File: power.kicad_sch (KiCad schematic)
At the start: 12 parts, among them J1 USB4215-03-A, U3 NCP1117 3.3, U4 USBLC6-2SC6

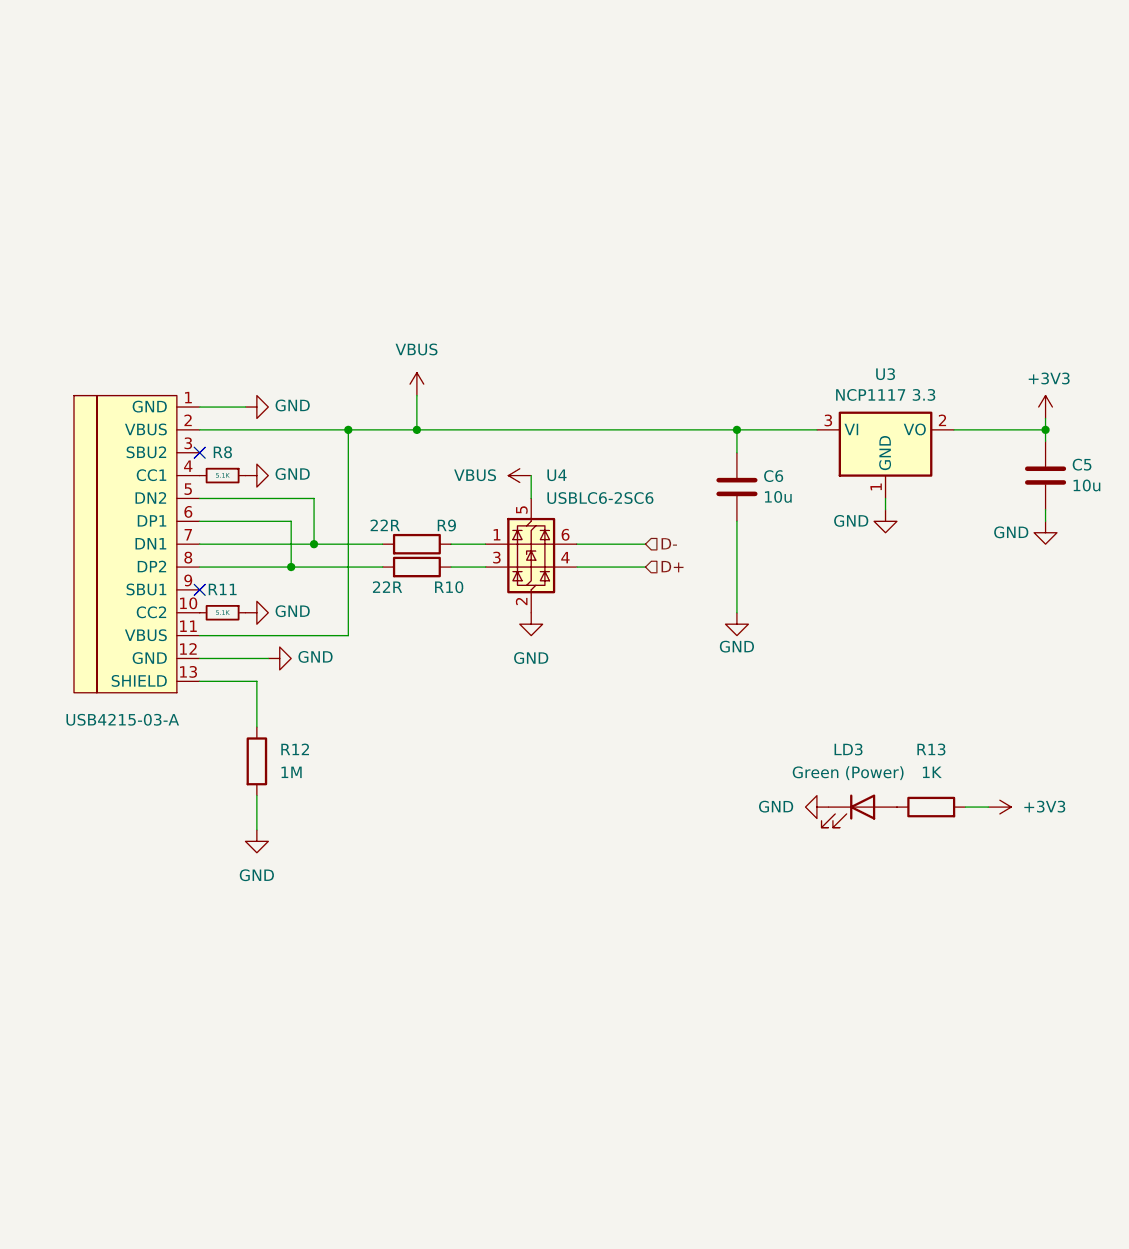
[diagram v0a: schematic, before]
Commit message: WIP
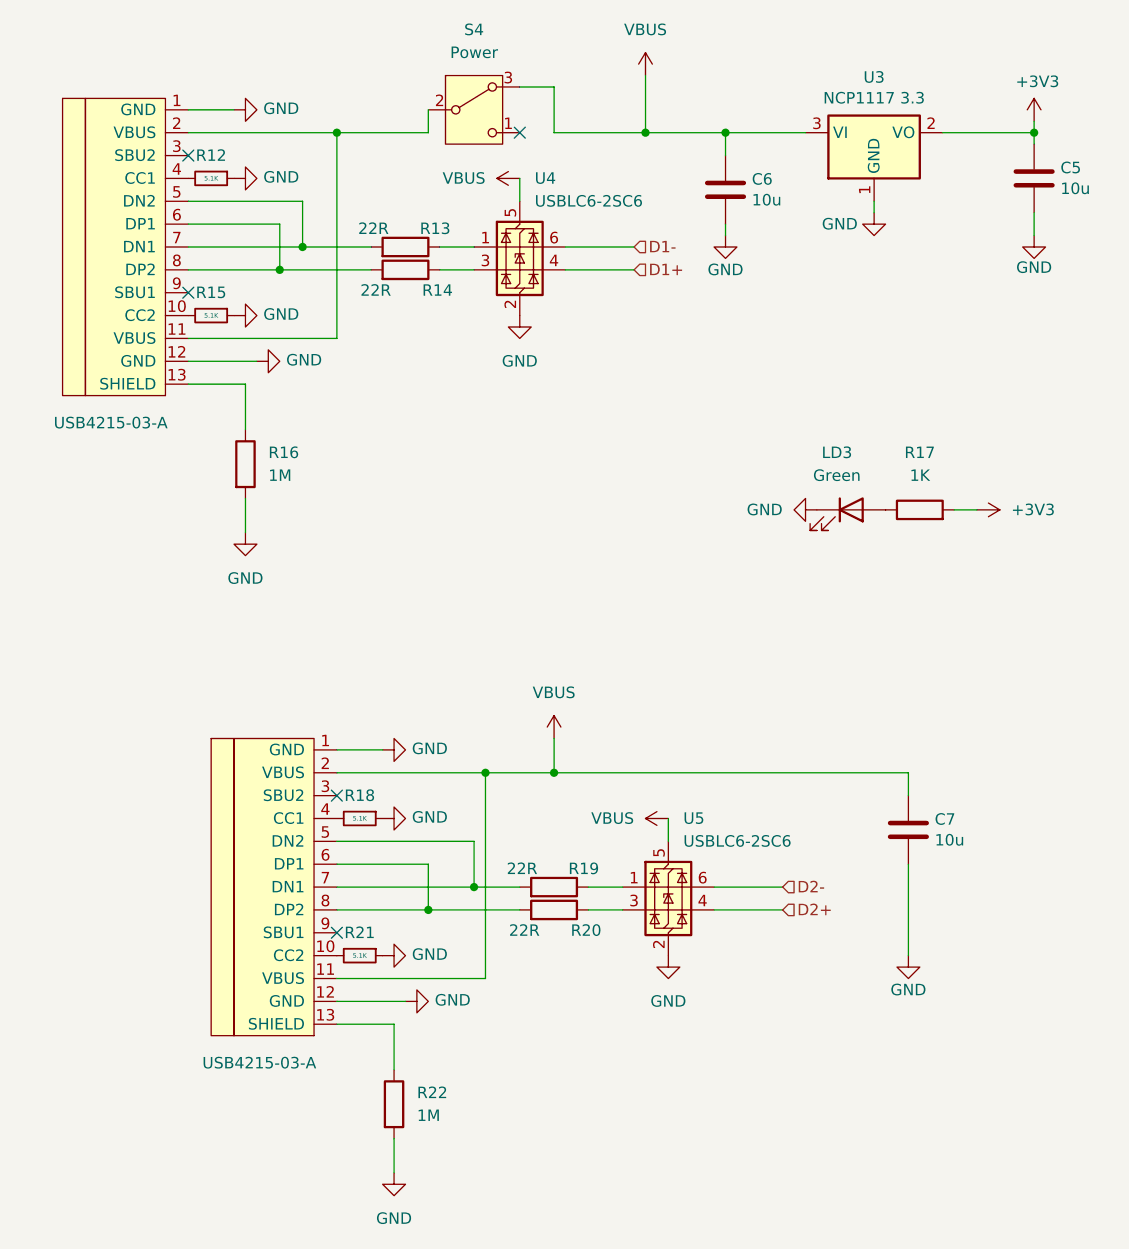
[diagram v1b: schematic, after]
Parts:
- added C7: 10u, FRANK:Capacitor (0805), symbol Device:C
- added J2: USB4215-03-A, FRANK:USB Type C, symbol FRANK:USB-C
- added R18, R21: 5.1K, FRANK:Resistor (0805), symbol Device:R_Small
- added R19, R20: 22R, FRANK:Resistor (0805), symbol Device:R
- added R22: 1M, FRANK:Resistor (0805), symbol Device:R
- added S4: Power, FRANK:Switch (MSK12C02), symbol Switch:SW_SPDT_321
- added U5: USBLC6-2SC6, FRANK:SOT-23-6, symbol Power_Protection:USBLC6-2SC6
- LD3: value Green (Power) -> Green
- U4: symbol Power_Protection:USBLC6-2SC6 -> FRANK:USBLC6-2SC6; AliExpress (none) -> https://vi.aliexpress.com/item/1005006883533480.html
- renumbered R8 to R12, R9 to R13, R10 to R14, R11 to R15, R12 to R16, R13 to R17
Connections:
- net GND: now also C7.2, J2.1 (GND), J2.12 (GND), R18.1, R21.1, R22.2, U5.2 (GND)
- net VBUS: now also C7.1, J2.11 (VBUS), J2.2 (VBUS), S4.3 (A), U5.5 (VBUS); no longer J1.11 (VBUS), J1.2 (VBUS)
- net D+ renamed D1+
- net D- renamed D1-
- new net: J1.11 (VBUS), J1.2 (VBUS), S4.2 (B)
- new net: J2.13 (SHIELD), R22.1
- new net: J2.4 (CC1), R18.2
- new net: R19.1, U5.1 (I/O1)
- new net: R20.1, U5.3 (I/O2)
- new net: J2.5 (DN2), J2.7 (DN1), R19.2
- new net: J2.6 (DP1), J2.8 (DP2), R20.2
- new net: J2.10 (CC2), R21.2
- new net D2+: U5.4 (I/O2)
- new net D2-: U5.6 (I/O1)
- no-connect marks 2 -> 5
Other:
- moved on the sheet: C5, C6, LD3, R12, R13, R14, R15, R16, R17, U3, U4

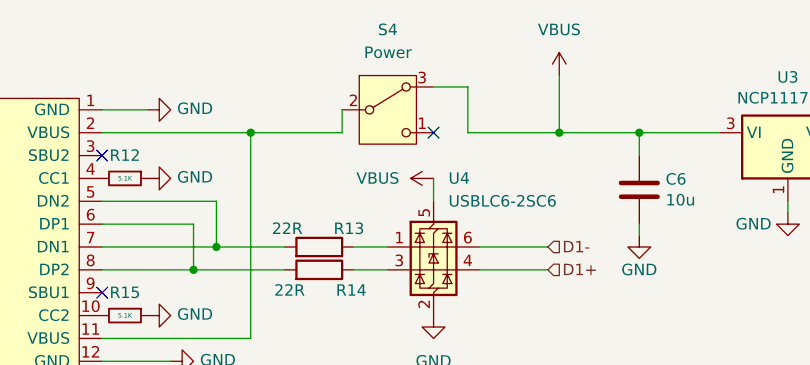
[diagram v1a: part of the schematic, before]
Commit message: Rev 1.05 WIP
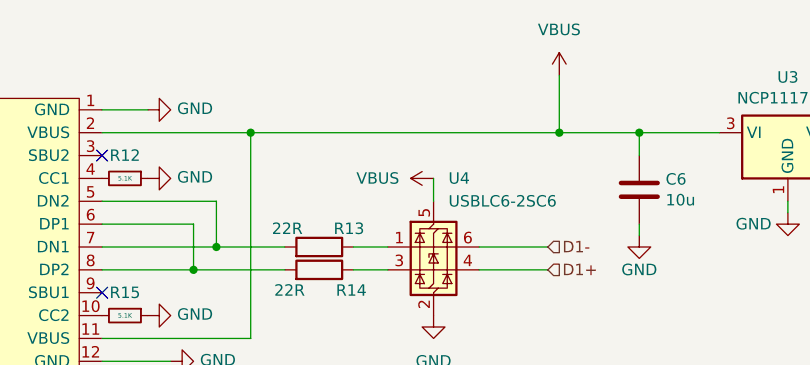
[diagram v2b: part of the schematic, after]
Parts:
- removed S4: Power, FRANK:Switch (MSK12C02), symbol Switch:SW_SPDT_321
- C5, C6, C7: footprint FRANK:Capacitor (0805) -> FRANK:Capacitor (0603)
- R12, R13, R14, R15, R16, R17, R18, R19, R20, R21, R22: footprint FRANK:Resistor (0805) -> FRANK:Resistor (0603)
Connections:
- net VBUS: now also J1.11 (VBUS), J1.2 (VBUS)
- no-connect marks 5 -> 4
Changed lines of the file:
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@@
 	)
 	(no_connect
-		(at 147.32 44.45)
-	)
-	(no_connect
 		(at 110.49 62.23)
 	)
@@
 	(wire
 		(pts
-			(xy 151.13 39.37) (xy 151.13 44.45)
-		)
-		(stroke
-			(width 0)
-			(type default)
-		)
-	)
-	(wire
-		(pts
 			(xy 163.83 120.65) (xy 163.83 123.19)
 		)
@@
 	(wire
 		(pts
-			(xy 127 44.45) (xy 137.16 44.45)
+			(xy 127 44.45) (xy 161.29 44.45)
 		)
 		(stroke
@@
 	(wire
 		(pts
-			(xy 151.13 44.45) (xy 161.29 44.45)
-		)
-		(stroke
-			(width 0)
-			(type default)
-		)
-	)
-	(wire
-		(pts
 			(xy 127 128.27) (xy 142.24 128.27)
 		)
@@
 	(wire
 		(pts
-			(xy 137.16 41.91) (xy 137.16 44.45)
-		)
-		(stroke
-			(width 0)
-			(type default)
-		)
-	)
-	(wire
-		(pts
 			(xy 168.91 128.27) (xy 176.53 128.27)
 		)
@@
 	(wire
 		(pts
-			(xy 147.32 39.37) (xy 151.13 39.37)
-		)
-		(stroke
-			(width 0)
-			(type default)
-		)
-	)
-	(wire
-		(pts
 			(xy 186.69 52.07) (xy 186.69 53.34)
 		)
@@
 	)
 	(symbol
-		(lib_id "Switch:SW_SPDT_321")
-		(at 142.24 41.91 0)
-		(unit 1)
-		(exclude_from_sim no)
-		(in_bom yes)
-		(on_board yes)
-		(dnp no)
-		(fields_autoplaced yes)
-		(property "Reference" "S4"
-			(at 142.24 33.02 0)
-			(effects
-				(font
-					(size 1.27 1.27)
-				)
-			)
-		)
-		(property "Value" "Power"
-			(at 142.24 35.56 0)
-			(effects
-				(font
-					(size 1.27 1.27)
-				)
-			)
-		)
-		(property "Footprint" "FRANK:Switch (MSK12C02)"
-			(at 142.24 52.07 0)
-			(effects
-				(font
-					(size 1.27 1.27)
-				)
-				(hide yes)
-			)
-		)
-		(property "Datasheet" "https://parts4laptops.eu/en/microbuttons/3300-microbutton-tact-switch-ts-1233-33x33x15mm-smt-mounting.html"
-			(at 142.24 49.53 0)
-			(effects
-				(font
-					(size 1.27 1.27)
-				)
-				(hide yes)
-			)
-		)
-		(property "Description" "Switch, single pole double throw"
-			(at 142.24 41.91 0)
-			(effects
-				(font
-					(size 1.27 1.27)
-				)
-				(hide yes)
-			)
-		)
-		(pin "2"
-		)
-		(pin "1"
-		)
-		(pin "3"
-		)
-		(instances
-			(project "echo"
-				(path "/8c0b3d8b-46d3-4173-ab1e-a61765f77d61/4ea27ee4-1edc-4e10-ab5a-91b9933087c0"
-					(reference "S4")
-					(unit 1)
-				)
-			)
-		)
-	)
-	(symbol
 		(lib_name "GND_5")
 		(lib_id "power:GND")
@@
 			)
 		)
-		(property "Footprint" "FRANK:Resistor (0805)"
+		(property "Footprint" "FRANK:Resistor (0603)"
 			(at 131.572 152.4 90)
 			(effects
@@
 			)
 		)
-		(property "Footprint" "FRANK:Capacitor (0805)"
+		(property "Footprint" "FRANK:Capacitor (0603)"
 			(at 191.4652 125.73 0)
 			(effects
@@
 			)
 		)
-		(property "Footprint" "FRANK:Resistor (0805)"
+		(property "Footprint" "FRANK:Resistor (0603)"
 			(at 134.62 58.928 90)
 			(effects
@@
 			)
 		)
-		(property "Footprint" "FRANK:Resistor (0805)"
+		(property "Footprint" "FRANK:Resistor (0603)"
 			(at 129.54 120.65 0)
 			(effects
@@
 			)
 		)
-		(property "Footprint" "FRANK:Capacitor (0805)"
+		(property "Footprint" "FRANK:Capacitor (0603)"
 			(at 205.4352 53.34 0)
 			(effects
@@
 			)
 		)
-		(property "Footprint" "FRANK:Capacitor (0805)"
+		(property "Footprint" "FRANK:Capacitor (0603)"
 			(at 171.1452 54.61 0)
 			(effects
@@
 			)
 		)
-		(property "Footprint" "FRANK:Resistor (0805)"
+		(property "Footprint" "FRANK:Resistor (0603)"
 			(at 191.77 88.138 90)
 			(effects
@@
 			)
 		)
-		(property "Footprint" "FRANK:Resistor (0805)"
+		(property "Footprint" "FRANK:Resistor (0603)"
 			(at 113.03 64.77 0)
 			(effects
@@
 			)
 		)
-		(property "Footprint" "FRANK:Resistor (0805)"
+		(property "Footprint" "FRANK:Resistor (0603)"
 			(at 113.03 49.53 0)
 			(effects
@@
 			)
 		)
-		(property "Footprint" "FRANK:Resistor (0805)"
+		(property "Footprint" "FRANK:Resistor (0603)"
 			(at 134.62 61.468 90)
 			(effects
@@
 			)
 		)
-		(property "Footprint" "FRANK:Resistor (0805)"
+		(property "Footprint" "FRANK:Resistor (0603)"
 			(at 151.13 130.048 90)
 			(effects
@@
 			)
 		)
-		(property "Footprint" "FRANK:Resistor (0805)"
+		(property "Footprint" "FRANK:Resistor (0603)"
 			(at 151.13 132.588 90)
 			(effects
@@
 			)
 		)
-		(property "Footprint" "FRANK:Resistor (0805)"
+		(property "Footprint" "FRANK:Resistor (0603)"
 			(at 115.062 81.28 90)
 			(effects
@@
 			)
 		)
-		(property "Footprint" "FRANK:Resistor (0805)"
+		(property "Footprint" "FRANK:Resistor (0603)"
 			(at 129.54 135.89 0)
 			(effects

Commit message: HW Revision 1.05
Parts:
- LD3: footprint FRANK:LED (0805) -> FRANK:LED (0603)
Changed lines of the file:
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@@
 			)
 		)
-		(property "Footprint" "FRANK:LED (0805)"
+		(property "Footprint" "FRANK:LED (0603)"
 			(at 184.15 86.36 0)
 			(effects
@@
 	)
 	(symbol
+		(lib_name "R_Small_3")
 		(lib_id "Device:R_Small")
 		(at 129.54 120.65 270)
@@
 			)
 		)
-		(property "Datasheet" "https://www.vishay.com/docs/28952/mcs0402at-mct0603at-mcu0805at-mca1206at.pdf"
+		(property "Datasheet" "~"
 			(at 129.54 120.65 0)
 			(effects
@@
 			)
 		)
-		(property "Description" ""
+		(property "Description" "Resistor, small symbol"
 			(at 129.54 120.65 0)
 			(effects
@@
 	)
 	(symbol
+		(lib_name "R_Small_2")
 		(lib_id "Device:R_Small")
 		(at 113.03 64.77 270)
@@
 			)
 		)
-		(property "Datasheet" "https://www.vishay.com/docs/28952/mcs0402at-mct0603at-mcu0805at-mca1206at.pdf"
+		(property "Datasheet" "~"
 			(at 113.03 64.77 0)
 			(effects
@@
 			)
 		)
-		(property "Description" ""
+		(property "Description" "Resistor, small symbol"
 			(at 113.03 64.77 0)
 			(effects
@@
 	)
 	(symbol
+		(lib_name "R_Small_1")
 		(lib_id "Device:R_Small")
 		(at 113.03 49.53 270)
@@
 			)
 		)
-		(property "Datasheet" "https://www.vishay.com/docs/28952/mcs0402at-mct0603at-mcu0805at-mca1206at.pdf"
+		(property "Datasheet" "~"
 			(at 113.03 49.53 0)
 			(effects
@@
 			)
 		)
-		(property "Description" ""
+		(property "Description" "Resistor, small symbol"
 			(at 113.03 49.53 0)
 			(effects
@@
 			)
 		)
-		(property "Datasheet" "https://www.vishay.com/docs/28952/mcs0402at-mct0603at-mcu0805at-mca1206at.pdf"
+		(property "Datasheet" "~"
 			(at 129.54 135.89 0)
 			(effects
@@
 			)
 		)
-		(property "Description" ""
+		(property "Description" "Resistor, small symbol"
 			(at 129.54 135.89 0)
 			(effects
